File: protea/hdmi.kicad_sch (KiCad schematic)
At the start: 10 parts, among them J5 HDMI Female

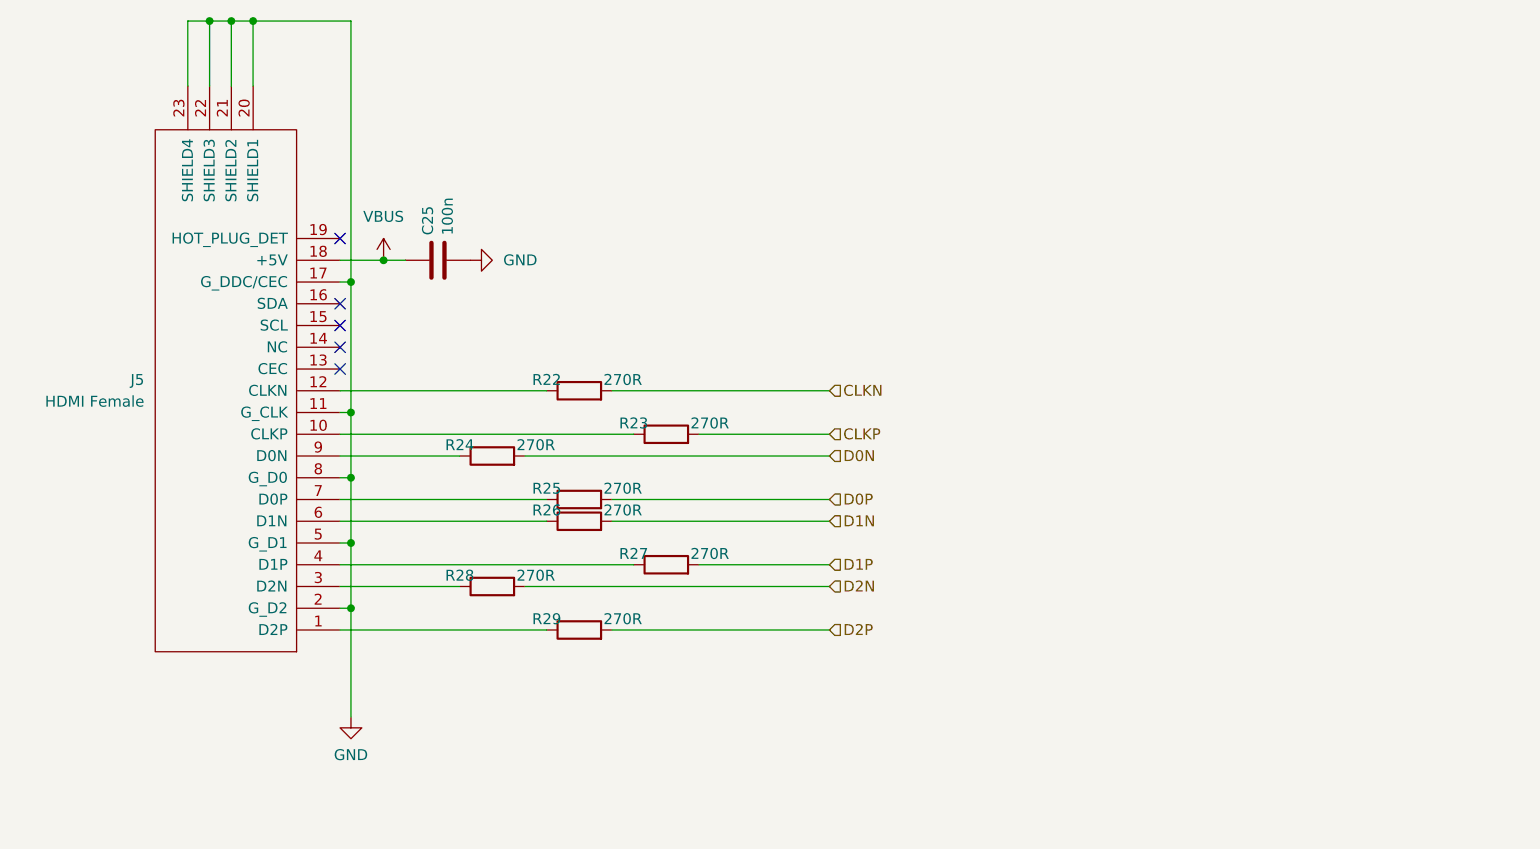
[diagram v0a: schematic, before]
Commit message: Protea HW 2.06
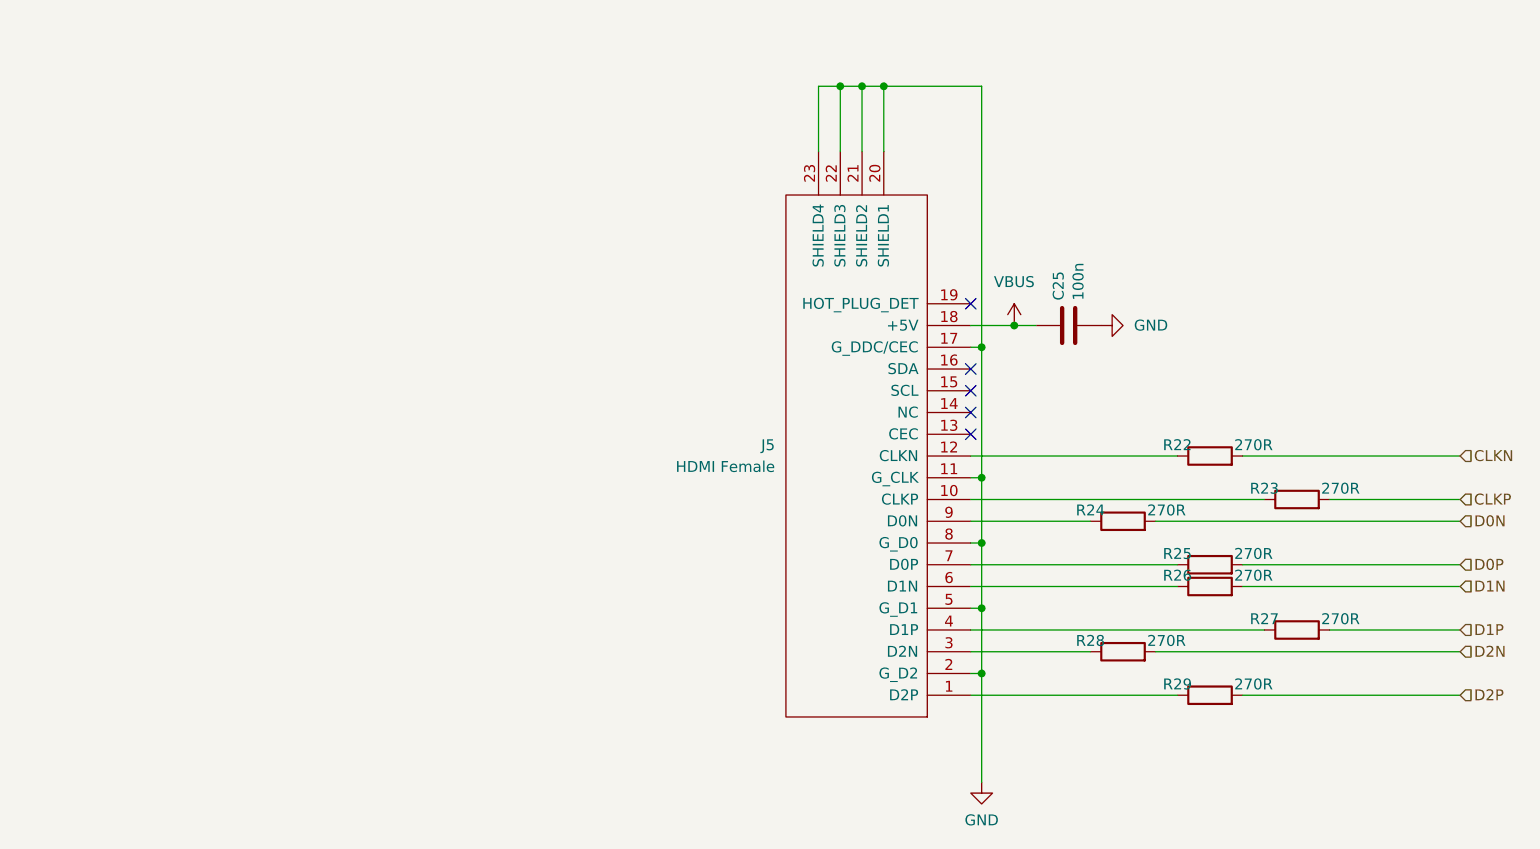
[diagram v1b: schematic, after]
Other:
- moved on the sheet: C25, J5, R22, R23, R24, R25, R26, R27, R28, R29
